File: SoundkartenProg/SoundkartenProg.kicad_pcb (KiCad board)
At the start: 2 copper layers, 17 x 23.5 mm, 5 parts, among them J1 TTL, J2 Soundkarte, J3 Messgerät, J4 12-16V, U1 74HC14

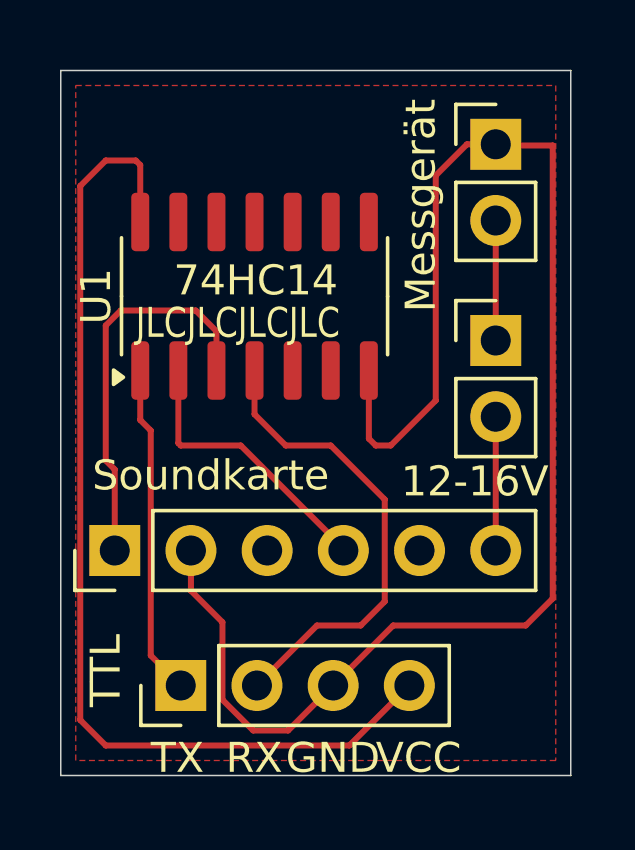
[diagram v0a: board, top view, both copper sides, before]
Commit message: kostenoptimierung
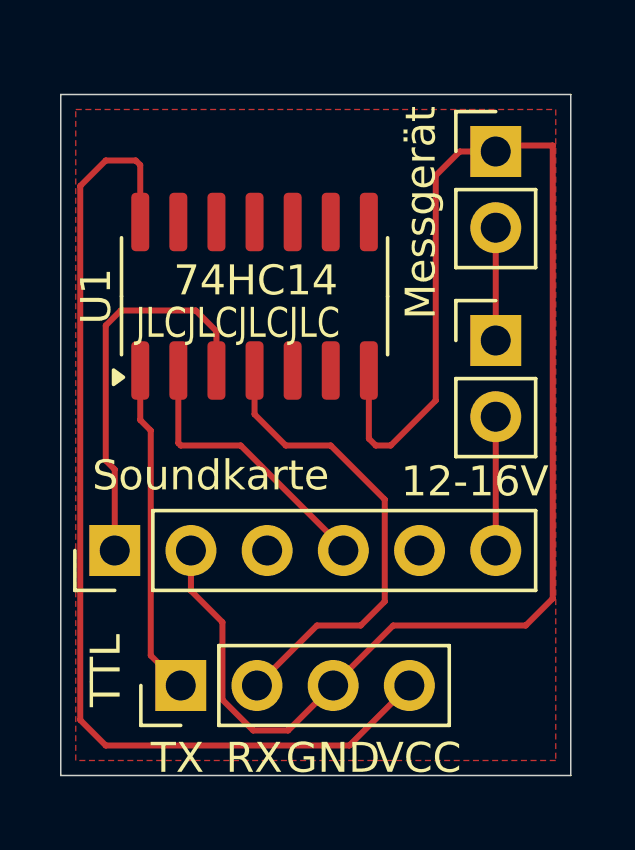
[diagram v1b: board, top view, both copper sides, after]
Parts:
- moved J3 0.24 mm to (132.5, 89.2)
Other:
- board size 17 x 23.5 mm -> 17 x 22.7 mm
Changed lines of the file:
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@@
 	(footprint "Connector_PinHeader_2.54mm:PinHeader_1x02_P2.54mm_Vertical"
 		(layer "F.Cu")
-		(at 132.5 88.96)
+		(at 132.5 89.2)
 		(descr "Through hole straight pin header, 1x02, 2.54mm pitch, single row")
 		(tags "Through hole pin header THT 1x02 2.54mm single row")
@@
 	)
 	(gr_rect
-		(start 118 86.5)
+		(start 118 87.3)
 		(end 135 110)
 		(stroke
@@
 		)
 	)
+	(dimension
+		(type aligned)
+		(layer "User.1")
+		(pts
+			(xy 118 86.5) (xy 135 86.5)
+		)
+		(height -2.7)
+		(gr_text "17,0000 mm"
+			(at 126.5 82.65 0)
+			(layer "User.1")
+			(effects
+				(font
+					(size 1 1)
+					(thickness 0.15)
+				)
+			)
+		)
+		(format
+			(prefix "")
+			(suffix "")
+			(units 3)
+			(units_format 1)
+			(precision 4)
+		)
+		(style
+			(thickness 0.1)
+			(arrow_length 1.27)
+			(text_position_mode 0)
+			(extension_height 0.58642)
+			(extension_offset 0.5) keep_text_aligned)
+	)
+	(dimension
+		(type aligned)
+		(layer "User.1")
+		(pts
+			(xy 135 110) (xy 135 87.3)
+		)
+		(height 3.4)
+		(gr_text "22,7000 mm"
+			(at 137.25 98.65 90)
+			(layer "User.1")
+			(effects
+				(font
+					(size 1 1)
+					(thickness 0.15)
+				)
+			)
+		)
+		(format
+			(prefix "")
+			(suffix "")
+			(units 3)
+			(units_format 1)
+			(precision 4)
+		)
+		(style
+			(thickness 0.1)
+			(arrow_length 1.27)
+			(text_position_mode 0)
+			(extension_height 0.58642)
+			(extension_offset 0.5) keep_text_aligned)
+	)
 	(segment
 		(start 121 98.5)
@@
 	)
 	(segment
-		(start 132.54 89)
-		(end 132.5 88.96)
+		(start 128.5 99)
+		(end 129 99)
+		(width 0.2)
+		(layer "F.Cu")
+		(net 10)
+	)
+	(segment
+		(start 129 99)
+		(end 130.5 97.5)
+		(width 0.2)
+		(layer "F.Cu")
+		(net 10)
+	)
+	(segment
+		(start 123.39 104.89)
+		(end 123.39 107.476346)
+		(width 0.2)
+		(layer "F.Cu")
+		(net 10)
+	)
+	(segment
+		(start 122.34 102.5)
+		(end 122.34 103.84)
+		(width 0.2)
+		(layer "F.Cu")
+		(net 10)
+	)
+	(segment
+		(start 131.3 89.2)
+		(end 132.5 89.2)
+		(width 0.2)
+		(layer "F.Cu")
+		(net 10)
+	)
+	(segment
+		(start 132.7 89)
+		(end 132.5 89.2)
+		(width 0.2)
+		(layer "F.Cu")
+		(net 10)
+	)
+	(segment
+		(start 134.4 104.1)
+		(end 134.4 89)
+		(width 0.2)
+		(layer "F.Cu")
+		(net 10)
+	)
+	(segment
+		(start 125.58 108.5)
+		(end 127.08 107)
+		(width 0.2)
+		(layer "F.Cu")
+		(net 10)
+	)
+	(segment
+		(start 127.08 107)
+		(end 129.08 105)
+		(width 0.2)
+		(layer "F.Cu")
+		(net 10)
+	)
+	(segment
+		(start 130.5 97.5)
+		(end 130.5 90)
+		(width 0.2)
+		(layer "F.Cu")
+		(net 10)
+	)
+	(segment
+		(start 128.27 98.77)
+		(end 128.5 99)
+		(width 0.2)
+		(layer "F.Cu")
+		(net 10)
+	)
+	(segment
+		(start 128.27 96.5)
+		(end 128.27 98.77)
+		(width 0.2)
+		(layer "F.Cu")
+		(net 10)
+	)
+	(segment
+		(start 122.34 103.84)
+		(end 123.39 104.89)
+		(width 0.2)
+		(layer "F.Cu")
+		(net 10)
+	)
+	(segment
+		(start 134.4 89)
+		(end 132.7 89)
+		(width 0.2)
+		(layer "F.Cu")
+		(net 10)
+	)
+	(segment
+		(start 130.5 90)
+		(end 131.3 89.2)
+		(width 0.2)
+		(layer "F.Cu")
+		(net 10)
+	)
+	(segment
+		(start 123.39 107.476346)
+		(end 124.413654 108.5)
+		(width 0.2)
+		(layer "F.Cu")
+		(net 10)
+	)
+	(segment
+		(start 129.08 105)
+		(end 133.5 105)
+		(width 0.2)
+		(layer "F.Cu")
+		(net 10)
+	)
+	(segment
+		(start 124.413654 108.5)
+		(end 125.58 108.5)
 		(width 0.2)
 		(layer "F.Cu")
@@
 	)
 	(segment
-		(start 129.08 105)
-		(end 133.5 105)
-		(width 0.2)
-		(layer "F.Cu")
-		(net 10)
-	)
-	(segment
-		(start 123.39 104.89)
-		(end 123.39 107.476346)
-		(width 0.2)
-		(layer "F.Cu")
-		(net 10)
-	)
-	(segment
-		(start 122.34 102.5)
-		(end 122.34 103.84)
-		(width 0.2)
-		(layer "F.Cu")
-		(net 10)
-	)
-	(segment
-		(start 128.5 99)
-		(end 129 99)
-		(width 0.2)
-		(layer "F.Cu")
-		(net 10)
-	)
-	(segment
-		(start 127.08 107)
-		(end 129.08 105)
-		(width 0.2)
-		(layer "F.Cu")
-		(net 10)
-	)
-	(segment
-		(start 130.5 97.5)
-		(end 130.5 90)
-		(width 0.2)
-		(layer "F.Cu")
-		(net 10)
-	)
-	(segment
-		(start 129 99)
-		(end 130.5 97.5)
-		(width 0.2)
-		(layer "F.Cu")
-		(net 10)
-	)
-	(segment
-		(start 130.5 90)
-		(end 131.54 88.96)
-		(width 0.2)
-		(layer "F.Cu")
-		(net 10)
-	)
-	(segment
-		(start 125.58 108.5)
-		(end 127.08 107)
-		(width 0.2)
-		(layer "F.Cu")
-		(net 10)
-	)
-	(segment
-		(start 122.34 103.84)
-		(end 123.39 104.89)
-		(width 0.2)
-		(layer "F.Cu")
-		(net 10)
-	)
-	(segment
-		(start 123.39 107.476346)
-		(end 124.413654 108.5)
-		(width 0.2)
-		(layer "F.Cu")
-		(net 10)
-	)
-	(segment
-		(start 124.413654 108.5)
-		(end 125.58 108.5)
-		(width 0.2)
-		(layer "F.Cu")
-		(net 10)
-	)
-	(segment
-		(start 128.27 96.5)
-		(end 128.27 98.77)
-		(width 0.2)
-		(layer "F.Cu")
-		(net 10)
-	)
-	(segment
-		(start 134.4 104.1)
-		(end 134.4 89)
-		(width 0.2)
-		(layer "F.Cu")
-		(net 10)
-	)
-	(segment
-		(start 131.54 88.96)
-		(end 132.5 88.96)
-		(width 0.2)
-		(layer "F.Cu")
-		(net 10)
-	)
-	(segment
-		(start 128.27 98.77)
-		(end 128.5 99)
-		(width 0.2)
-		(layer "F.Cu")
-		(net 10)
-	)
-	(segment
-		(start 134.4 89)
-		(end 132.54 89)
-		(width 0.2)
-		(layer "F.Cu")
-		(net 10)
-	)
-	(segment
 		(start 128 105)
 		(end 128.8 104.2)
@@
 	)
 	(segment
-		(start 132.5 91.5)
+		(start 132.5 91.74)
 		(end 132.5 95.5)
 		(width 0.2)
@@
 		(polygon
 			(pts
-				(xy 118.5 87) (xy 134.5 87) (xy 134.5 109.5) (xy 118.5 109.5)
-			)
-		)
+				(xy 118.5 87.8) (xy 134.5 87.8) (xy 134.5 109.5) (xy 118.5 109.5)
+			)
+		)
